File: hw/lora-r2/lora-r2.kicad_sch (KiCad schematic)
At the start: 9 parts, among them J1 Conn_Coaxial, J2 SWD, J3 Conn_02x08_Odd_Even, U1 Pico_1_PCB

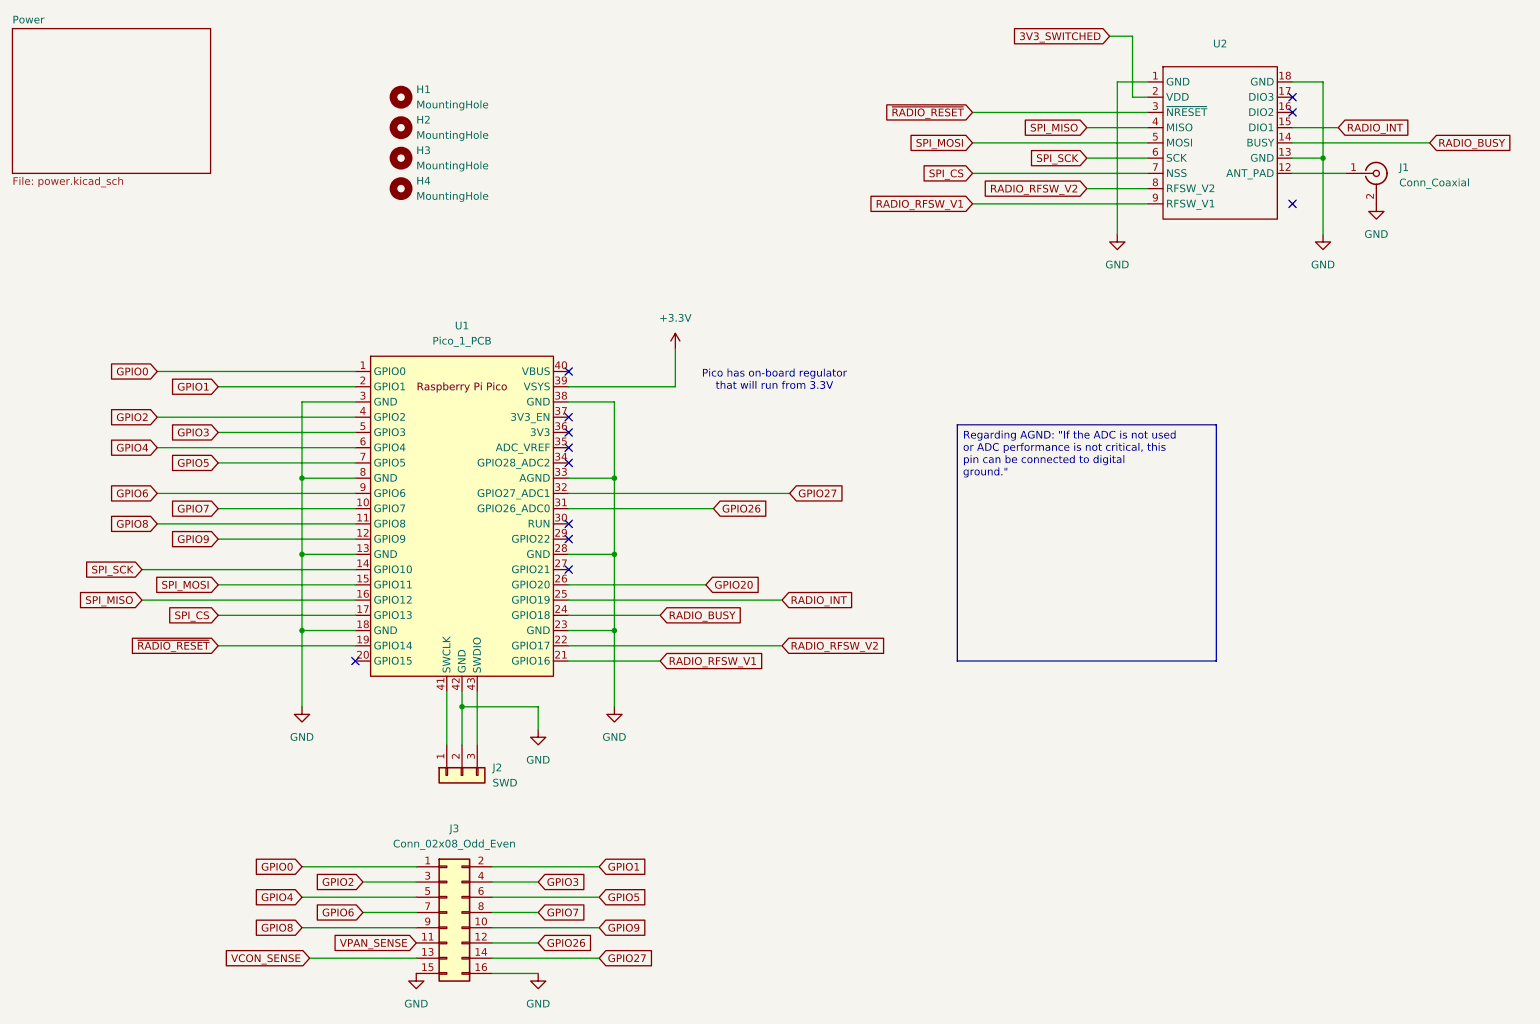
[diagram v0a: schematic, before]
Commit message: Making progress on layout
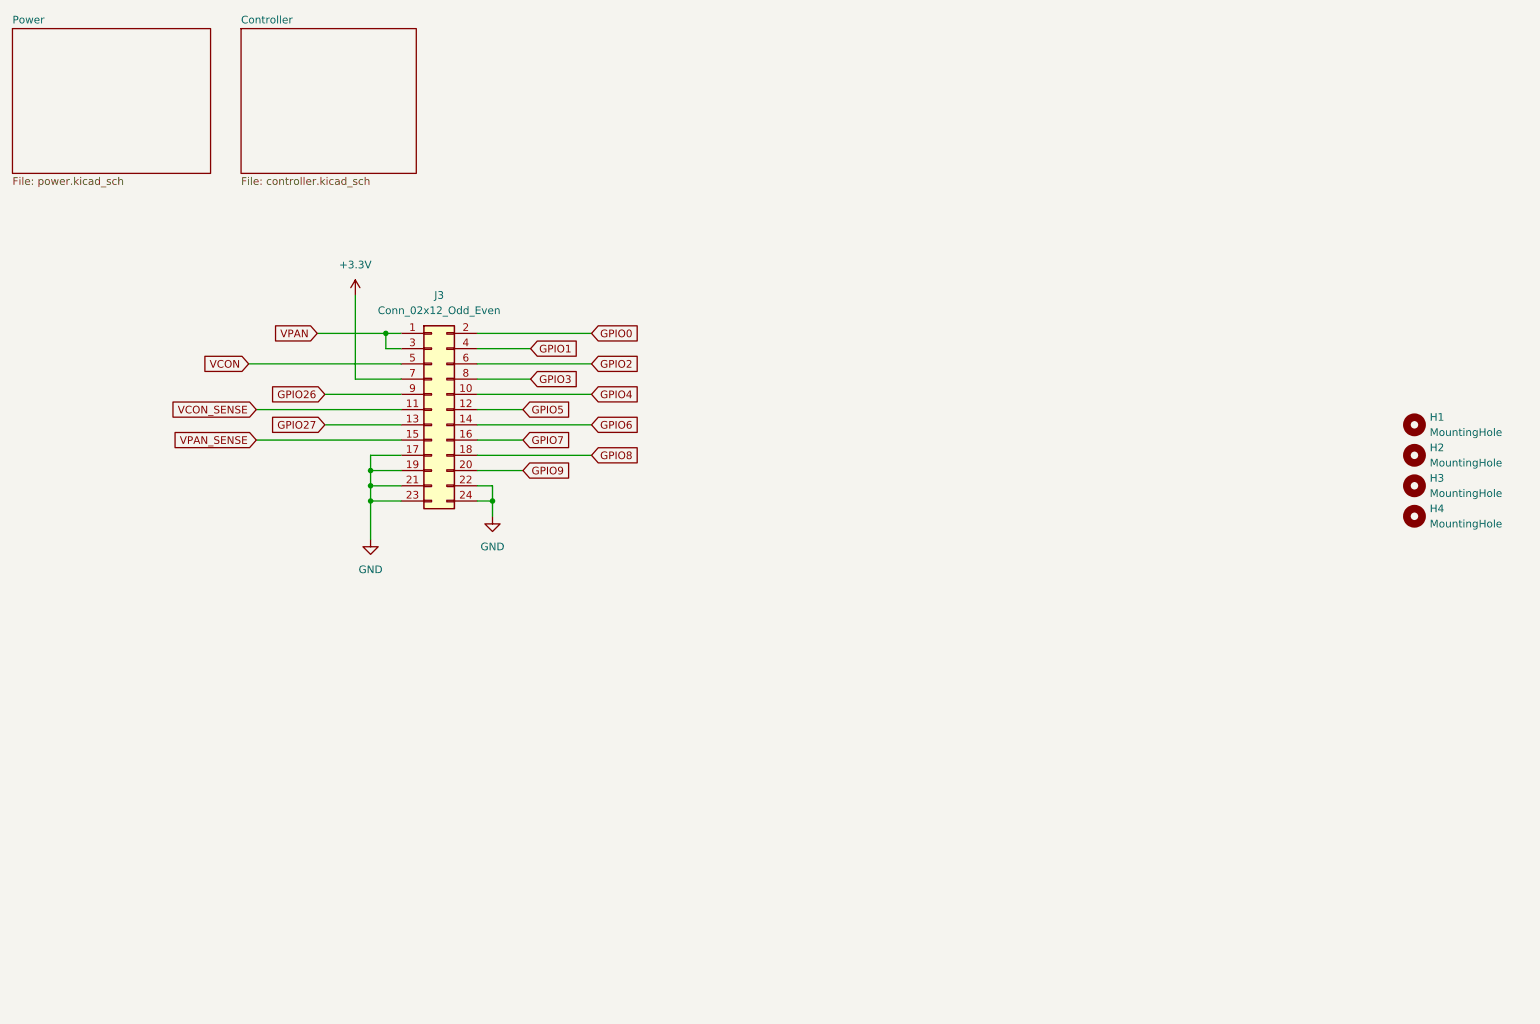
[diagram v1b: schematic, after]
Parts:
- removed J1: Conn_Coaxial, Connector_Coaxial:SMA_Amphenol_132134_Vertical, symbol Connector:Conn_Coaxial
- removed J2: SWD, Connector_PinHeader_2.54mm:PinHeader_1x03_P2.54mm_Vertical, symbol Connector_Generic:Conn_01x03
- removed J3: Conn_02x08_Odd_Even, Connector_PinHeader_2.54mm:PinHeader_2x08_P2.54mm_Vertical, symbol Connector_Generic:Conn_02x08_Odd_Even
- removed U1: Pico_1_PCB, bruce-footprints:RPi_Pico_SMD, symbol symbol-library-1:Pico_1_PCB
- removed U2: ~, bruce-footprints:RYLR689-LoRa-Module, symbol symbol-library-1:RYLR689_LoRa_Module
- added J3: Conn_02x12_Odd_Even, Connector_PinHeader_2.54mm:PinHeader_2x12_P2.54mm_Vertical, symbol Connector_Generic:Conn_02x12_Odd_Even
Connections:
- net +3.3V: now also J3.7 (Pin_7)
- net GND: now also J3.17 (Pin_17), J3.19 (Pin_19), J3.21 (Pin_21), J3.22 (Pin_22), J3.23 (Pin_23), J3.24 (Pin_24)
- net GPIO0: now also J3.2 (Pin_2)
- net GPIO1: now also J3.4 (Pin_4)
- net GPIO2: now also J3.6 (Pin_6)
- net GPIO26: now also J3.9 (Pin_9)
- net GPIO27: now also J3.13 (Pin_13)
- net GPIO3: now also J3.8 (Pin_8)
- net GPIO4: now also J3.10 (Pin_10)
- net GPIO5: now also J3.12 (Pin_12)
- net GPIO6: now also J3.14 (Pin_14)
- net GPIO7: now also J3.16 (Pin_16)
- net GPIO8: now also J3.18 (Pin_18)
- net GPIO9: now also J3.20 (Pin_20)
- net VCON_SENSE: now also J3.11 (Pin_11)
- net VPAN_SENSE: now also J3.15 (Pin_15)
- new net VCON: J3.5 (Pin_5)
- new net VPAN: J3.1 (Pin_1), J3.3 (Pin_3)
- no-connect marks 12 -> 0
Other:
- added sheet Controller (controller.kicad_sch)
- note removed: "Pico has on-board regulator that will run from 3.3V"
- moved on the sheet: H1, H2, H3, H4
